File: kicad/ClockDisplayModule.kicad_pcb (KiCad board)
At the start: 2 copper layers, 91.4 x 58.4 mm, 43 parts, among them IC101 ATMEGA8-P, P101 CONN_02X03, P102 CONN_01X05, P201 CONN_01X06, P202 CONN_01X07, P203 CONN_01X06, P204 CONN_01X07, Q201 BC856BS, Q202 BC856BS, Q203 BC856BS, U201 SN74LS138, U202 74HC4511

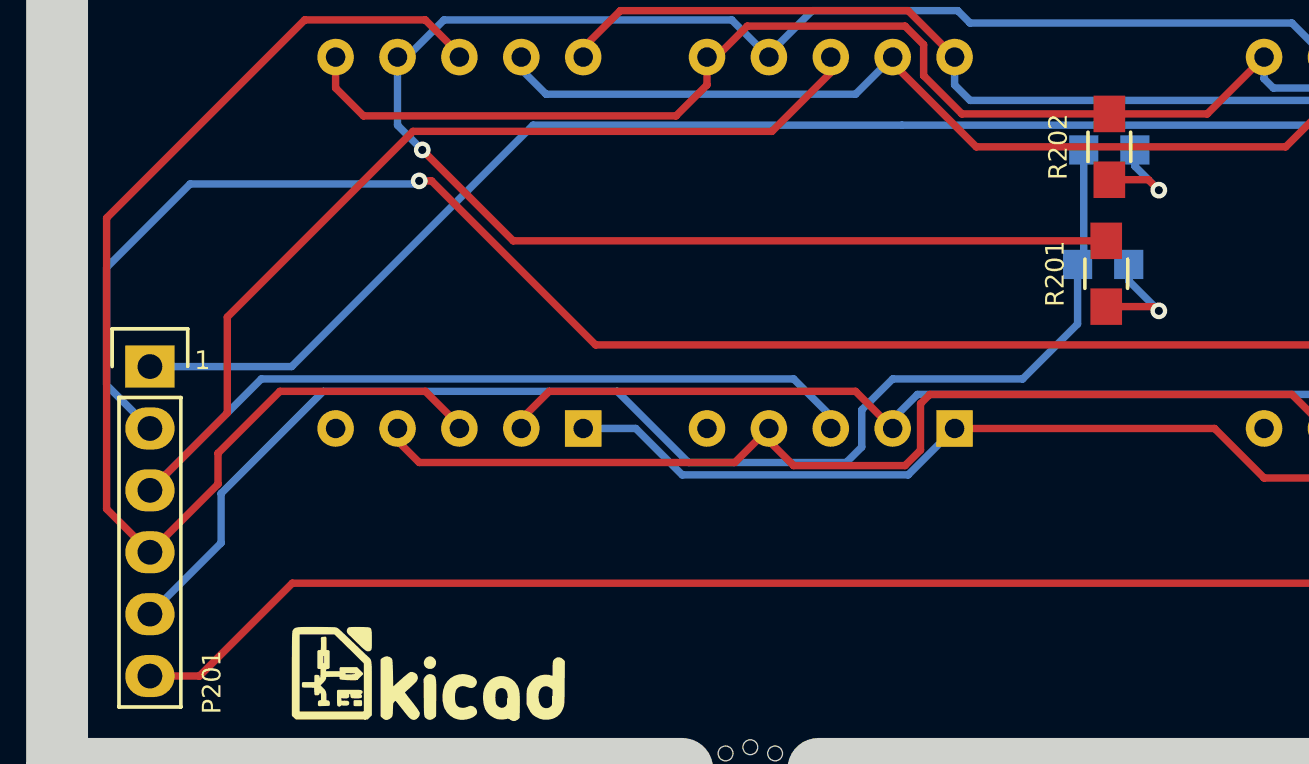
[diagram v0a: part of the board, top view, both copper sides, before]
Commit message: Changes to the gerbers
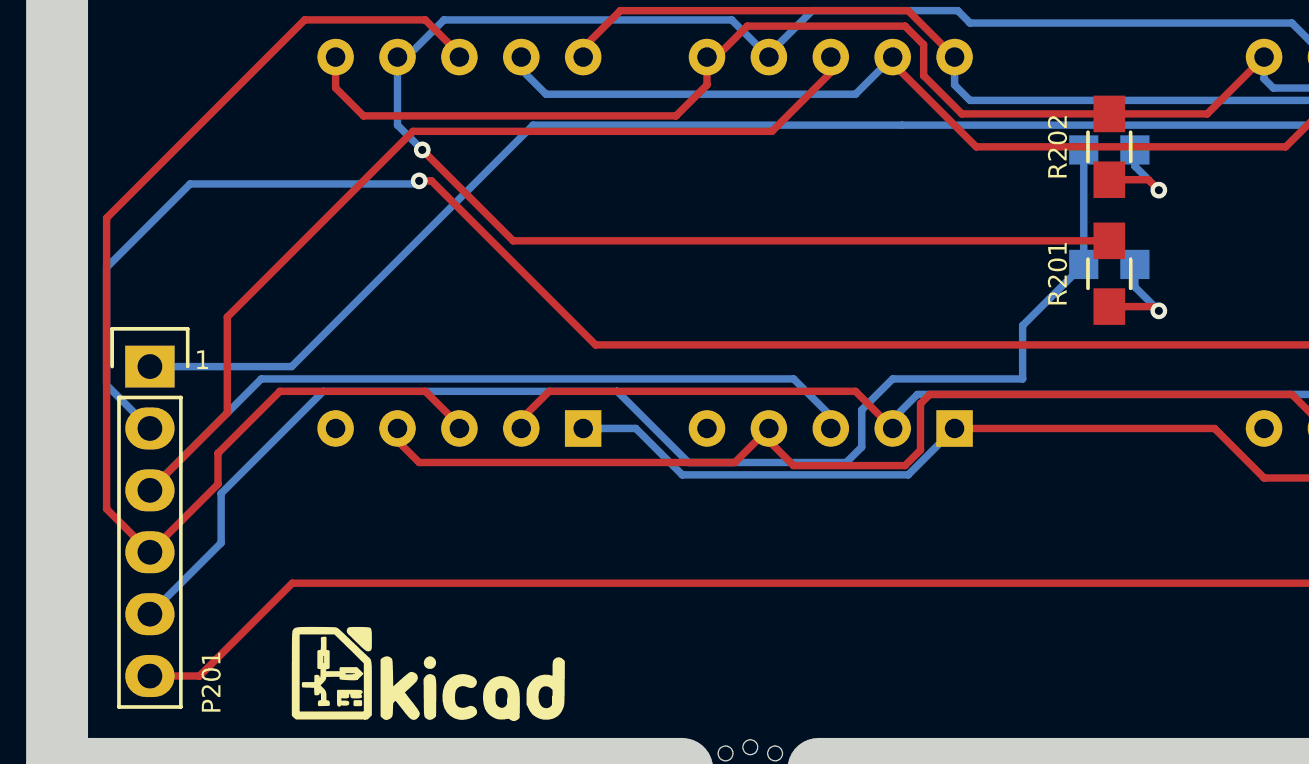
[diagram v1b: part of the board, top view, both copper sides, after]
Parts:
- moved D201 0.25 mm to (158.8, 56.8)
- moved R201 0.13 mm to (158.8, 57.1)
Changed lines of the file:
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@@
     (pad_drill 0.6)
     (pad_to_mask_clearance 0)
+    (pad_to_paste_clearance 0.0254)
     (aux_axis_origin 0 0)
     (visible_elements FFFEFF7F)
@@
   )
   (module LEDs:LED-0805 (layer B.Cu)
-    (at 158.496 56.769)
+    (at 158.75 56.769)
     (descr "LED 0805 smd package")
     (tags "LED 0805 SMD")
@@
   )
   (module Resistors_SMD:R_0805_HandSoldering (layer F.Cu)
-    (at 158.623 57.15 90)
+    (at 158.75 57.15 90)
     (descr "Resistor SMD 0805, hand soldering")
     (tags "resistor 0805")
@@
   (segment (start 197.057 54.69) (end 200.787 58.42) (width 0.3048) (layer B.Cu) (net 6))
   (segment (start 200.787 58.42) (end 201.93 58.42) (width 0.3048) (layer B.Cu) (net 6))
-  (segment (start 158.623 55.8) (end 134.286 55.8) (width 0.3048) (layer F.Cu) (net 6))
+  (segment (start 158.75 55.8) (end 134.286 55.8) (width 0.3048) (layer F.Cu) (net 6) (status 10))
   (segment (start 134.286 55.8) (end 130.556 52.07) (width 0.3048) (layer F.Cu) (net 6))
   (via (at 130.556 52.07) (size 0.6858) (drill 0.3302) (layers F.Cu B.Cu) (net 6))
@@
   (segment (start 177.165 92.075) (end 177.8 92.71) (width 0.3048) (layer B.Cu) (net 13))
   (via (at 177.165 92.075) (size 0.6858) (drill 0.3302) (layers F.Cu B.Cu) (net 13))
-  (segment (start 159.54502 56.769) (end 159.54502 57.43702) (width 0.3048) (layer B.Cu) (net 14))
-  (segment (start 159.54502 57.43702) (end 160.782 58.674) (width 0.3048) (layer B.Cu) (net 14))
+  (segment (start 159.79902 56.769) (end 159.79902 57.69102) (width 0.3048) (layer B.Cu) (net 14))
   (via (at 160.782 58.674) (size 0.6858) (drill 0.3302) (layers F.Cu B.Cu) (net 14))
   (segment (start 160.782 58.674) (end 160.608 58.5) (width 0.3048) (layer F.Cu) (net 14))
-  (segment (start 160.608 58.5) (end 158.623 58.5) (width 0.3048) (layer F.Cu) (net 14))
+  (segment (start 160.608 58.5) (end 158.75 58.5) (width 0.3048) (layer F.Cu) (net 14) (status 20))
+  (segment (start 159.79902 57.69102) (end 160.782 58.674) (width 0.3048) (layer B.Cu) (net 14))
+  (segment (start 157.70098 56.769) (end 157.70098 52.07) (width 0.3048) (layer B.Cu) (net 15))
+  (segment (start 155.194 61.468) (end 155.194 59.27598) (width 0.3048) (layer B.Cu) (net 15))
+  (segment (start 155.194 61.468) (end 149.86 61.468) (width 0.3048) (layer B.Cu) (net 15))
+  (segment (start 149.86 61.468) (end 148.59 62.738) (width 0.3048) (layer B.Cu) (net 15))
+  (segment (start 148.59 62.738) (end 148.59 64.262) (width 0.3048) (layer B.Cu) (net 15))
+  (segment (start 148.59 64.262) (end 147.955 64.897) (width 0.3048) (layer B.Cu) (net 15))
+  (segment (start 147.955 64.897) (end 141.478 64.897) (width 0.3048) (layer B.Cu) (net 15))
+  (segment (start 141.478 64.897) (end 138.557 61.976) (width 0.3048) (layer B.Cu) (net 15))
+  (segment (start 119.38 71.12) (end 122.301 68.199) (width 0.3048) (layer B.Cu) (net 15))
+  (segment (start 122.301 66.167) (end 122.301 68.199) (width 0.3048) (layer B.Cu) (net 15))
+  (segment (start 126.492 61.976) (end 122.301 66.167) (width 0.3048) (layer B.Cu) (net 15))
   (segment (start 138.557 61.976) (end 126.492 61.976) (width 0.3048) (layer B.Cu) (net 15))
-  (segment (start 126.492 61.976) (end 122.301 66.167) (width 0.3048) (layer B.Cu) (net 15))
-  (segment (start 122.301 66.167) (end 122.301 68.199) (width 0.3048) (layer B.Cu) (net 15))
-  (segment (start 122.301 68.199) (end 119.38 71.12) (width 0.3048) (layer B.Cu) (net 15))
-  (segment (start 157.44698 56.769) (end 157.44698 59.21502) (width 0.3048) (layer B.Cu) (net 15))
-  (segment (start 141.478 64.897) (end 138.557 61.976) (width 0.3048) (layer B.Cu) (net 15))
-  (segment (start 147.955 64.897) (end 141.478 64.897) (width 0.3048) (layer B.Cu) (net 15))
-  (segment (start 148.59 64.262) (end 147.955 64.897) (width 0.3048) (layer B.Cu) (net 15))
-  (segment (start 148.59 62.738) (end 148.59 64.262) (width 0.3048) (layer B.Cu) (net 15))
-  (segment (start 149.86 61.468) (end 148.59 62.738) (width 0.3048) (layer B.Cu) (net 15))
-  (segment (start 155.194 61.468) (end 149.86 61.468) (width 0.3048) (layer B.Cu) (net 15))
-  (segment (start 157.44698 59.21502) (end 155.194 61.468) (width 0.3048) (layer B.Cu) (net 15))
-  (segment (start 157.70098 52.07) (end 157.70098 56.515) (width 0.3048) (layer B.Cu) (net 15))
-  (segment (start 157.70098 56.515) (end 157.44698 56.769) (width 0.1524) (layer B.Cu) (net 15))
+  (segment (start 155.194 59.27598) (end 157.70098 56.769) (width 0.3048) (layer B.Cu) (net 15))
+  (segment (start 157.95498 56.515) (end 157.70098 56.769) (width 0.1524) (layer B.Cu) (net 15) (status 30))
   (segment (start 159.79902 52.07) (end 159.79902 52.73802) (width 0.3048) (layer B.Cu) (net 16))
   (segment (start 159.79902 52.73802) (end 160.782 53.721) (width 0.3048) (layer B.Cu) (net 16))
